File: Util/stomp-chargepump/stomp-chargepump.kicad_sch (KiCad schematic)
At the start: 15 parts, among them J1 to-effect, J2 to-effect, J3 from-top-jacks, J4 to-effect, U1 MAX1044

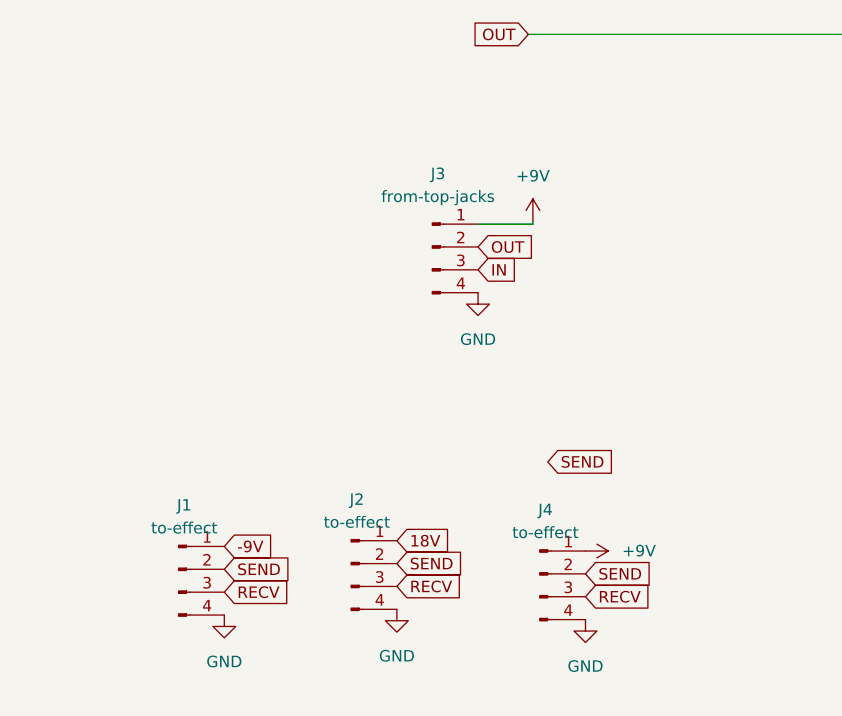
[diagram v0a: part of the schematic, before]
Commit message: missing files
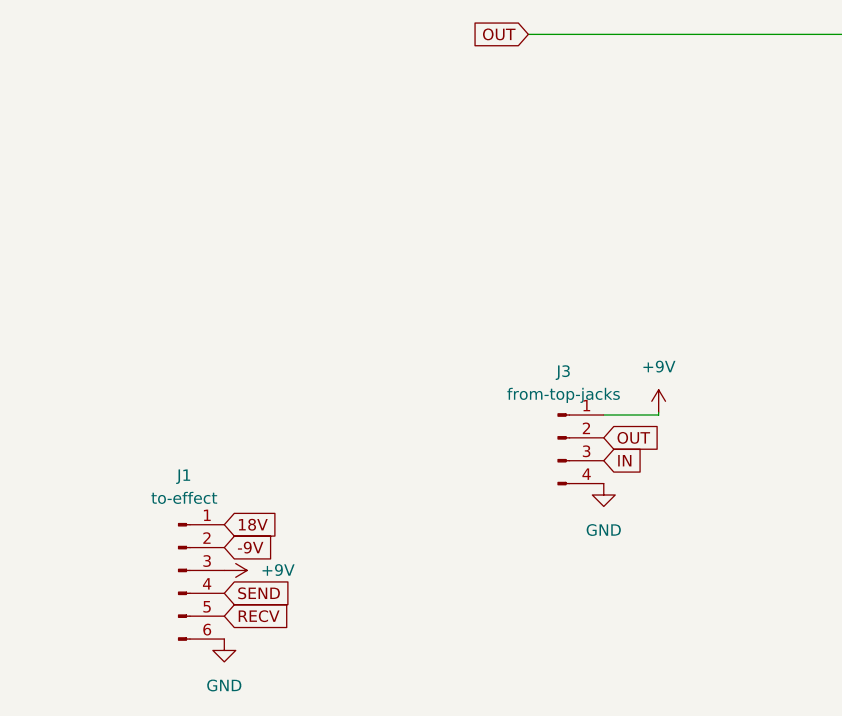
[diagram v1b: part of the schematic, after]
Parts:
- removed J2, J4: to-effect, Connector_PinHeader_2.54mm:PinHeader_1x04_P2.54mm_Vertical, symbol Connector:Conn_01x04_Pin
- J1: footprint Connector_PinHeader_2.54mm:PinHeader_1x04_P2.54mm_Vertical -> Connector_PinHeader_2.54mm:PinHeader_1x06_P2.54mm_Vertical; symbol Connector:Conn_01x04_Pin -> Connector:Conn_01x06_Pin
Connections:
- net +9V: now also J1.3 (Pin_3)
- net -9V: now also J1.2 (Pin_2); no longer J1.1 (Pin_1)
- net 18V: now also J1.1 (Pin_1)
- net GND: now also J1.6 (Pin_6); no longer J1.4 (Pin_4)
- net RECV: now also J1.5 (Pin_5); no longer J1.3 (Pin_3)
- net SEND: now also J1.4 (Pin_4); no longer J1.2 (Pin_2)
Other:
- moved on the sheet: J3
